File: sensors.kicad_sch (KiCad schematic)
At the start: 17 parts, among them Q1 TEMT6000X01, U6 MAX4466EXK, U7 BME280

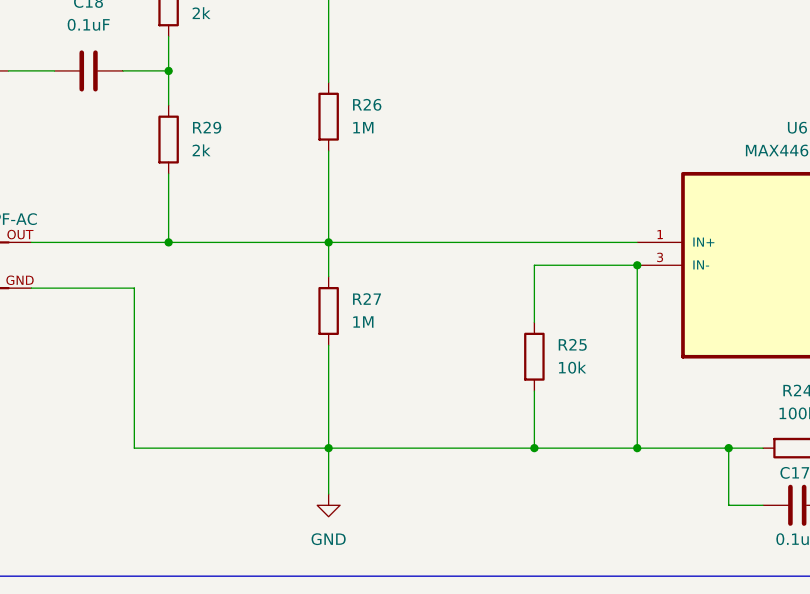
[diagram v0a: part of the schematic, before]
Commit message: Fixed Audio Amp Circuit
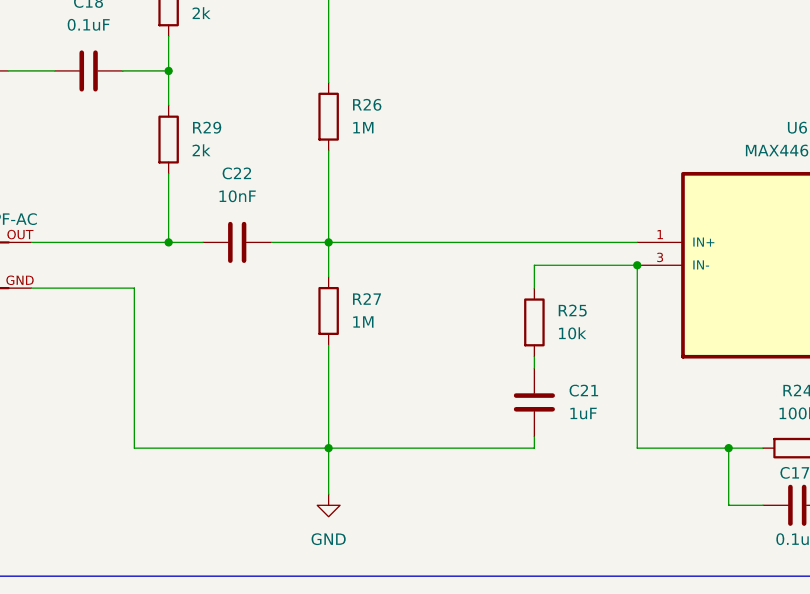
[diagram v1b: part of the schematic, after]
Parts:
- added C21: 1uF, Resistor_SMD:R_0805_2012Metric, symbol Device:C
- added C22: 10nF, Resistor_SMD:R_0805_2012Metric, symbol Device:C
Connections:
- net GND: now also C21.2; no longer C17.1, R24.2, R25.1, R25.2, U6.3 (IN-)
- net at R26.2, R27.1, U6.1 (IN+): now also C22.2; no longer MK1.OUT, R29.2
- new net: C17.1, R24.2, R25.1, U6.3 (IN-)
- new net: C21.1, R25.2
- new net: C22.1, MK1.OUT, R29.2
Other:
- moved on the sheet: R25
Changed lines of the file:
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@@
-	)
-	(junction
-		(at 95.25 162.56)
-		(diameter 0)
-		(color 0 0 0 0)
 	)
 	(junction
@@
 	)
 	(junction
-		(at 54.61 139.7)
-		(diameter 0)
-		(color 0 0 0 0)
-	)
-	(junction
 		(at 55.88 35.56)
 		(diameter 0)
@@
 	)
 	(junction
-		(at 106.68 162.56)
-		(diameter 0)
-		(color 0 0 0 0)
-	)
-	(junction
 		(at 162.56 134.62)
 		(diameter 0)
@@
 		(color 0 0 0 0)
 	)
+	(junction
+		(at 54.61 139.7)
+		(diameter 0)
+		(color 0 0 0 0)
+	)
 	(no_connect
 		(at 189.23 46.99)
@@
 	(wire
 		(pts
-			(xy 95.25 148.59) (xy 95.25 142.24)
+			(xy 95.25 144.78) (xy 95.25 142.24)
 		)
 		(stroke
@@
 	(wire
 		(pts
-			(xy 95.25 162.56) (xy 95.25 156.21)
-		)
-		(stroke
-			(width 0)
-			(type default)
-		)
-	)
-	(wire
-		(pts
 			(xy 54.61 109.22) (xy 54.61 101.6)
 		)
@@
 	(wire
 		(pts
+			(xy 54.61 139.7) (xy 58.42 139.7)
+		)
+		(stroke
+			(width 0)
+			(type default)
+		)
+	)
+	(wire
+		(pts
 			(xy 205.74 30.48) (xy 205.74 36.83)
 		)
@@
 	(wire
 		(pts
-			(xy 54.61 139.7) (xy 72.39 139.7)
-		)
-		(stroke
-			(width 0)
-			(type default)
-		)
-	)
-	(wire
-		(pts
 			(xy 162.56 127) (xy 162.56 134.62)
 		)
@@
 	(wire
 		(pts
-			(xy 95.25 162.56) (xy 106.68 162.56)
-		)
-		(stroke
-			(width 0)
-			(type default)
-		)
-	)
-	(wire
-		(pts
 			(xy 59.69 60.96) (xy 55.88 60.96)
 		)
@@
 	(wire
 		(pts
+			(xy 66.04 139.7) (xy 72.39 139.7)
+		)
+		(stroke
+			(width 0)
+			(type default)
+		)
+	)
+	(wire
+		(pts
 			(xy 36.83 44.45) (xy 36.83 35.56)
 		)
@@
 	(wire
 		(pts
+			(xy 95.25 161.29) (xy 95.25 162.56)
+		)
+		(stroke
+			(width 0)
+			(type default)
+		)
+	)
+	(wire
+		(pts
 			(xy 72.39 129.54) (xy 72.39 139.7)
+		)
+		(stroke
+			(width 0)
+			(type default)
+		)
+	)
+	(wire
+		(pts
+			(xy 95.25 152.4) (xy 95.25 153.67)
 		)
 		(stroke
@@
 	(symbol
 		(lib_id "Device:R")
-		(at 95.25 152.4 0)
+		(at 95.25 148.59 0)
 		(unit 1)
 		(exclude_from_sim no)
@@
 		(fields_autoplaced yes)
 		(property "Reference" "R25"
-			(at 97.79 151.1299 0)
+			(at 97.79 147.3199 0)
 			(effects
 				(font
@@
 		)
 		(property "Value" "10k"
-			(at 97.79 153.6699 0)
+			(at 97.79 149.8599 0)
 			(effects
 				(font
@@
 		)
 		(property "Footprint" "Resistor_SMD:R_0805_2012Metric"
-			(at 93.472 152.4 90)
+			(at 93.472 148.59 90)
 			(effects
 				(font
@@
 		)
 		(property "Datasheet" "~"
-			(at 95.25 152.4 0)
+			(at 95.25 148.59 0)
 			(effects
 				(font
@@
 		)
 		(property "Description" "Resistor"
-			(at 95.25 152.4 0)
+			(at 95.25 148.59 0)
 			(effects
 				(font
@@
 	)
 	(symbol
+		(lib_id "Device:C")
+		(at 62.23 139.7 90)
+		(unit 1)
+		(exclude_from_sim no)
+		(in_bom yes)
+		(on_board yes)
+		(dnp no)
+		(fields_autoplaced yes)
+		(property "Reference" "C22"
+			(at 62.23 132.08 90)
+			(effects
+				(font
+					(size 1.27 1.27)
+				)
+			)
+		)
+		(property "Value" "10nF"
+			(at 62.23 134.62 90)
+			(effects
+				(font
+					(size 1.27 1.27)
+				)
+			)
+		)
+		(property "Footprint" "Resistor_SMD:R_0805_2012Metric"
+			(at 66.04 138.7348 0)
+			(effects
+				(font
+					(size 1.27 1.27)
+				)
+				(hide yes)
+			)
+		)
+		(property "Datasheet" "~"
+			(at 62.23 139.7 0)
+			(effects
+				(font
+					(size 1.27 1.27)
+				)
+				(hide yes)
+			)
+		)
+		(property "Description" "Unpolarized capacitor"
+			(at 62.23 139.7 0)
+			(effects
+				(font
+					(size 1.27 1.27)
+				)
+				(hide yes)
+			)
+		)
+		(pin "2"
+		)
+		(pin "1"
+		)
+		(instances
+			(project ""
+				(path "/8e18a6b6-2497-40ab-aacd-16656297d80d/0980fd62-4755-455b-bc26-b8079d26a0ec/ac745bbd-23e4-454a-ab24-96f5aa9d51bc"
+					(reference "C22")
+					(unit 1)
+				)
+			)
+		)
+	)
+	(symbol
 		(lib_id "Device:R")
 		(at 36.83 48.26 0)
@@
 					(unit 1)
 				)
+			)
+		)
+	)
+	(symbol
+		(lib_id "Device:C")
+		(at 95.25 157.48 0)
+		(unit 1)
+		(exclude_from_sim no)
+		(in_bom yes)
+		(on_board yes)
+		(dnp no)
+		(fields_autoplaced yes)
+		(property "Reference" "C21"
+			(at 99.06 156.2099 0)
+			(effects
+				(font
+					(size 1.27 1.27)
+				)
+				(justify left)
+			)
+		)
+		(property "Value" "1uF"
+			(at 99.06 158.7499 0)
+			(effects
+				(font
+					(size 1.27 1.27)
+				)
+				(justify left)
+			)
+		)
+		(property "Footprint" "Resistor_SMD:R_0805_2012Metric"
+			(at 96.2152 161.29 0)
+			(effects
+				(font
+					(size 1.27 1.27)
+				)
+				(hide yes)
+			)
+		)
+		(property "Datasheet" "~"
+			(at 95.25 157.48 0)
+			(effects
+				(font
+					(size 1.27 1.27)
+				)
+				(hide yes)
+			)
+		)
+		(property "Description" "Unpolarized capacitor"
+			(at 95.25 157.48 0)
+			(effects
+				(font
+					(size 1.27 1.27)
+				)
+				(hide yes)
+			)
+		)
+		(pin "2"
+		)
+		(pin "1"
+		)
+		(instances
+			(project ""
+				(path "/8e18a6b6-2497-40ab-aacd-16656297d80d/0980fd62-4755-455b-bc26-b8079d26a0ec/ac745bbd-23e4-454a-ab24-96f5aa9d51bc"
+					(reference "C21")
+					(unit 1)
+				)

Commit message: Fixed the Footprint assignment nonsense
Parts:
- C15, C16, C17, C18, C21, C22: footprint Resistor_SMD:R_0805_2012Metric -> Capacitor_SMD:C_0805_2012Metric
- MK1: footprint Resistor_SMD:R_0805_2012Metric -> CMC-5042PF-AC:CUI_CMC-5042PF-AC
- Q1: footprint Resistor_SMD:R_0805_2012Metric -> TEMT6000X01:TRANS_TEMT6000X01
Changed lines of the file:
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@@
 			)
 		)
-		(property "Footprint" "Resistor_SMD:R_0805_2012Metric"
+		(property "Footprint" "Capacitor_SMD:C_0805_2012Metric"
 			(at 128.27 167.9448 0)
 			(effects
@@
 			)
 		)
-		(property "Footprint" "Resistor_SMD:R_0805_2012Metric"
+		(property "Footprint" "Capacitor_SMD:C_0805_2012Metric"
 			(at 49.53 119.6848 0)
 			(effects
@@
 			)
 		)
-		(property "Footprint" "Resistor_SMD:R_0805_2012Metric"
+		(property "Footprint" "Capacitor_SMD:C_0805_2012Metric"
 			(at 66.04 138.7348 0)
 			(effects
@@
 			)
 		)
-		(property "Footprint" "Resistor_SMD:R_0805_2012Metric"
+		(property "Footprint" "Capacitor_SMD:C_0805_2012Metric"
 			(at 163.5252 144.78 0)
 			(effects
@@
 			)
 		)
-		(property "Footprint" "Resistor_SMD:R_0805_2012Metric"
+		(property "Footprint" "Capacitor_SMD:C_0805_2012Metric"
 			(at 100.0252 59.69 0)
 			(effects
@@
 			)
 		)
-		(property "Footprint" "Resistor_SMD:R_0805_2012Metric"
+		(property "Footprint" "CMC-5042PF-AC:CUI_CMC-5042PF-AC"
 			(at 31.75 142.24 0)
 			(effects
@@
 			)
 		)
-		(property "Footprint" "Resistor_SMD:R_0805_2012Metric"
+		(property "Footprint" "Capacitor_SMD:C_0805_2012Metric"
 			(at 96.2152 161.29 0)
 			(effects
@@
 			)
 		)
-		(property "Footprint" "Resistor_SMD:R_0805_2012Metric"
+		(property "Footprint" "TEMT6000X01:TRANS_TEMT6000X01"
 			(at 196.85 57.15 0)
 			(effects
